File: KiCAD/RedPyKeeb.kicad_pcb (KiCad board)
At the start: 4 copper layers, 482.6 x 183.4 mm, 340 parts, among them J0 Conn_01x04, J1 Conn_01x04, K0,0 KEYSW, K0,1 KEYSW, K0,2 KEYSW, K0,3 KEYSW, K0,4 KEYSW, K0,5 KEYSW, K1,0 KEYSW, K1,1 KEYSW, K1,2 KEYSW, K1,3 KEYSW, K1,4 KEYSW, K1,5 KEYSW, K10,0 KEYSW, K10,1 KEYSW, K10,2 KEYSW, K10,3 KEYSW, K10,4 KEYSW, K10,5 KEYSW, K11,0 KEYSW, K11,1 KEYSW, K11,2 KEYSW, K11,3 KEYSW, K11,4 KEYSW, K11,5 KEYSW, K12,0 KEYSW, K12,1 KEYSW, K12,2 KEYSW, K12,3 KEYSW, K13,1 KEYSW, K13,2 KEYSW, K14,0 KEYSW, K14,1 KEYSW, K14,3 KEYSW, K14,6 KEYSW, K15,0 KEYSW, K15,1 KEYSW, K15,3 KEYSW, K15,5 KEYSW, K15,6 KEYSW, K16,0 KEYSW, K16,1 KEYSW, K16,3 KEYSW, K16,4 KEYSW, K16,5 KEYSW, K16,6 KEYSW, K17,0 KEYSW, K17,1 KEYSW, K17,3 KEYSW, K17,4 KEYSW, K17,5 KEYSW, K17,6 KEYSW, K18,0 KEYSW, K18,1 KEYSW, K18,3 KEYSW, K18,4 KEYSW, K18,5 KEYSW, K18,6 KEYSW, K19,0 KEYSW, K19,1 KEYSW, K19,3 KEYSW, K19,4 KEYSW, K19,6 KEYSW, K2,0 KEYSW, K2,1 KEYSW, K2,2 KEYSW, K2,3 KEYSW, K2,4 KEYSW, K2,5 KEYSW, K20,0 KEYSW, K20,1 KEYSW, K3,0 KEYSW, K3,1 KEYSW, K3,2 KEYSW, K3,3 KEYSW, K3,4 KEYSW, K3,5 KEYSW, K4,0 KEYSW, K4,1 KEYSW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

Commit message: Update KiCAD files.
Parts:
- added C4: 0805B101K100CT, Capacitor_SMD:C_0805_2012Metric_Pad1.18x1.45mm_HandSolder, B.Cu at (452.6, 82.5)
- added C5: 0805B101K100CT, Capacitor_SMD:C_0805_2012Metric_Pad1.18x1.45mm_HandSolder, B.Cu at (438.0, 80.3)
- added C7: 0805B101K100CT, Capacitor_SMD:C_0805_2012Metric_Pad1.18x1.45mm_HandSolder, B.Cu at (438.1, 75.0)
- added J2: Conn_01x04, Connector_JST:JST_EH_S4B-EH_1x04_P2.50mm_Horizontal, F.Cu at (442.1, 51.3)
- added R1: APC0805B1K00N, Resistors_SMD:R_0805_HandSoldering, B.Cu at (458.1, 81.9)
- added R2: APC0805B1K00N, Resistors_SMD:R_0805_HandSoldering, B.Cu at (460.1, 81.9)
- added R3: ERJ-6RED2003V, Resistors_SMD:R_0805_HandSoldering, B.Cu at (460.2, 78.5)
- added R4: APC0805B1K00N, Resistors_SMD:R_0805_HandSoldering, B.Cu at (458.5, 74.0)
- added R5: APC0805B1K00N, Resistors_SMD:R_0805_HandSoldering, B.Cu at (456.6, 74.0)
- C1, C2: moved to F.Cu
- C3: moved to B.Cu
- C6: value EEE-FK1A102AL -> EEE-FN1C102UV
- D0,0, D0,1, D0,2, D0,3, D0,4, D0,5, D1,0, D1,1, D1,2, D1,3, D1,4, D1,5, D10,0, D10,1, D10,2, D10,3, D10,4, D10,5, D11,0, D11,1, D11,2, D11,3, D11,4, D11,5, D12,0, D12,1, D12,3, D13,1, D13,2, D14,0, D14,1, D14,3, D14,6, D15,0, D15,1, D15,3, D15,5, D15,6, D16,0, D16,1, D16,3, D16,4, D16,5, D16,6, D17,0, D17,1, D17,3, D17,4, D17,5, D17,6, D18,0, D18,1, D18,3, D18,4, D18,5, D18,6, D19,0, D19,1, D19,3, D19,4, D19,6, D2,0, D2,1, D2,2, D2,3, D2,4, D2,5, D20,0, D20,1, D3,0, D3,1, D3,2, D3,3, D3,4, D3,5, D4,0, D4,1, D4,2, D4,3, D4,4, D5,0, D5,1, D5,2, D5,3, D5,4, D6,0, D6,1, D6,2, D6,3, D6,4, D7,0, D7,1, D7,2, D7,3, D7,4, D8,0, D8,1, D8,2, D8,3, D8,4, D8,5, D9,0, D9,1, D9,2, D9,3, D9,4, D9,5: value D -> BAT54W-HG3-08
- K0,0, K0,1, K0,2, K0,3, K0,4, K0,5, K1,0, K1,1, K1,2, K1,3, K1,4, K1,5, K10,0, K10,1, K10,2, K10,3, K10,4, K10,5, K11,0, K11,1, K11,2, K11,3, K11,4, K11,5, K12,0, K12,1, K12,2, K12,3, K13,1, K13,2, K14,0, K14,1, K14,3, K14,6, K15,0, K15,1, K15,3, K15,5, K15,6, K16,0, K16,1, K16,3, K16,4, K16,5, K16,6, K17,0, K17,1, K17,3, K17,4, K17,5, K17,6, K18,0, K18,1, K18,3, K18,4, K18,5, K18,6, K19,0, K19,1, K19,3, K19,4, K19,6, K2,0, K2,1, K2,2, K2,3, K2,4, K2,5, K20,0, K20,1, K3,0, K3,1, K3,2, K3,3, K3,4, K3,5, K4,0, K4,1, K4,2, K4,3, K4,4, K5,0, K5,1, K5,2, K5,3, K5,4, K6,0, K6,1, K6,2, K6,3, K6,4, K7,0, K7,1, K7,2, K7,3, K7,4, K8,0, K8,1, K8,2, K8,3, K8,4, K8,5, K9,0, K9,1, K9,2, K9,3, K9,4, K9,5: value KEYSW -> ~
- LD0,0, LD0,1, LD0,2, LD0,3, LD0,4, LD0,5, LD1,0, LD1,1, LD1,2, LD1,3, LD1,4, LD1,5, LD10,0, LD10,1, LD10,2, LD10,3, LD10,4, LD10,5, LD11,0, LD11,1, LD11,2, LD11,3, LD11,4, LD11,5, LD12,0, LD12,1, LD12,2, LD12,3, LD13,1, LD13,2, LD14,0, LD14,1, LD14,3, LD14,6, LD15,0, LD15,1, LD15,3, LD15,5, LD15,6, LD16,0, LD16,1, LD16,3, LD16,4, LD16,5, LD16,6, LD17,0, LD17,1, LD17,3, LD17,4, LD17,5, LD17,6, LD17,7, LD18,0, LD18,1, LD18,3, LD18,4, LD18,5, LD18,6, LD18,7, LD19,0, LD19,1, LD19,3, LD19,4, LD19,6, LD19,7, LD2,0, LD2,1, LD2,2, LD2,3, LD2,4, LD2,5, LD20,0, LD20,1, LD20,7, LD3,0, LD3,1, LD3,2, LD3,3, LD3,4, LD3,5, LD4,0, LD4,1, LD4,2, LD4,3, LD4,4, LD5,0, LD5,1, LD5,2, LD5,3, LD5,4, LD6,0, LD6,1, LD6,2, LD6,3, LD6,4, LD7,0, LD7,1, LD7,2, LD7,3, LD7,4, LD8,0, LD8,1, LD8,2, LD8,3, LD8,4, LD8,5, LD9,0, LD9,1, LD9,2, LD9,3, LD9,4, LD9,5: value APA102-2020 -> APA102 2020
- U0: value USB_Pico -> ~
- U10: value PCA9306DP -> PCA9306DQER; footprint Package_SO:SO-8_3.9x4.9mm_P1.27mm -> Package_SO:SSOP-8_2.95x2.8mm_P0.65mm
- moved U10 375.7 mm to (455.4, 79.4)
- moved U11 374.3 mm to (443.8, 78.7)
- moved U0 348.4 mm to (431.9, 67.1)
- moved C6 346.7 mm to (491.4, 73.0)
- moved J0 344.5 mm to (486.9, 60.4)
- moved J1 339.7 mm to (480.7, 80.6), turned to 180 degrees
- moved C2 334.7 mm to (409.2, 84.2)
- moved U2 332.3 mm to (405.7, 84.3), turned to 270 degrees
- moved U1 36.6 mm to (107.4, 112.3), turned to 180 degrees
- moved U3 34.5 mm to (83.8, 86.1), turned to 270 degrees
- moved C1 33.6 mm to (107.8, 114.3), turned to 270 degrees
- moved C3 24.8 mm to (80.4, 86.5)
- moved K20,0 22.7 mm to (501.3, 102.5)
- moved LD20,0 22.7 mm to (501.3, 95.7)
- moved D17,0 22.7 mm to (435.6, 103.7)
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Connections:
- U10 pad 7: MAIN_VBUS -> Net-(C4-Pad2)
- U10 pad 8: MAIN_VBUS -> Net-(C4-Pad2)
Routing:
- net MAIN_VBUS: track 4476.7 -> 4998.0 mm, vias 47 -> 57
- net KEY_COL16: track 594.8 -> 181.5 mm
- net KEY_COL20: track 558.3 -> 149.0 mm
- net KEY_COL19: track 621.8 -> 214.2 mm
- net KEY_COL18: track 605.4 -> 200.1 mm
- net KEY_COL17: track 594.2 -> 190.0 mm
- net I2C_SDA0: track 60.3 -> 450.4 mm, vias 3 -> 5
- net I2C_SCL0: track 59.1 -> 447.0 mm, vias 4 -> 5
- net GNDPWR: track 3230.2 -> 3610.8 mm, vias 6 -> 9
- net PICO_33_REF: track 125.0 -> 497.8 mm, vias 1 -> 3
- net KEY_COL15: track 527.8 -> 178.2 mm
- net IO_INT0: track 46.6 -> 371.8 mm, vias 2 -> 4
- net KEY_COL14: track 507.4 -> 187.7 mm
- net IO_INT1: track 50.7 -> 367.3 mm, vias 2 -> 4
- net KEY_COL12: track 406.3 -> 146.0 mm, vias 2 -> 0
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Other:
- board size 482.6 x 183.4 mm -> 448.3 x 179.1 mm
- net class USB added: clearance 0.2, trace_width 0.4, via_dia 0.8, via_drill 0.4

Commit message: Update firmware and KiCAD files.
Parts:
- D12,2: value BAT54W-HG3-18 -> BAT54W-HG3-08
- J2: footprint Connector_JST:JST_EH_S4B-EH_1x04_P2.50mm_Horizontal -> Connector_JST:JST_EH_S7B-EH_1x07_P2.50mm_Horizontal
- U10: value PCA9306DQER -> PCA9306DP
- moved J2 2.95 mm to (445.0, 50.9)
- moved LD13,2 1.03 mm to (353.3, 140.7)
- moved LD0,4 1.03 mm to (100.2, 179.9)
- moved LD19,1 0.50 mm to (482.1, 121.5)
- moved LD0,2 0.35 mm to (93.1, 140.7)
- moved LD19,0 0.24 mm to (482.0, 95.6)
- moved LD17,0 0.12 mm to (443.4, 95.6)
- moved LD18,0 0.12 mm to (462.7, 95.6)
- moved LD20,0 0.11 mm to (501.3, 95.6)
- moved LD17,3 0.10 mm to (443.5, 140.7)
- moved LD18,3 0.10 mm to (462.8, 140.7)
- moved LD19,3 0.10 mm to (482.1, 140.7)
- moved LD0,0 0.08 mm to (88.5, 95.5)
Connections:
- U0 pad 21: Net-(J2-Pad4) -> Net-(U0-Pad21)
- U0 pad 22: Net-(J2-Pad3) -> Net-(J2-Pad5)
- U0 pad 24: Net-(J2-Pad2) -> Net-(J2-Pad3)
- U0 pad 25: Net-(J2-Pad1) -> Net-(J2-Pad4)
- U0 pad 26: Net-(U0-Pad26) -> Net-(J2-Pad6)
- U0 pad 27: Net-(U0-Pad27) -> Net-(J2-Pad7)
- U0 pad 36: Net-(U0-Pad36) -> Net-(J2-Pad1)
- U0 pad 38: Net-(U0-Pad38) -> Net-(J2-Pad2)
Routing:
- net MAIN_VBUS: track 4998.0 -> 4783.6 mm, vias 57 -> 56
- net GNDPWR: track 3610.8 -> 3540.1 mm
- net Net-(J2-Pad2): track 4.13 -> 37.3 mm
- net Net-(J2-Pad7): track 0.00 -> 28.9 mm
- net Net-(J2-Pad1): track 4.82 -> 29.0 mm
- net Net-(J2-Pad6): track 0.00 -> 24.1 mm
- net Net-(LD16,3-Pad2): track 30.4 -> 22.2 mm
- net Net-(J2-Pad5): track 0.00 -> 3.54 mm
- net Net-(J2-Pad4): track 4.11 -> 7.24 mm
- net Net-(LD17,0-Pad3): track 16.2 -> 17.6 mm
- net Net-(LD14,3-Pad3): track 16.2 -> 17.6 mm
- net Net-(LD14,1-Pad3): track 16.2 -> 17.6 mm
- net Net-(LD10,5-Pad4): track 21.1 -> 22.5 mm
- net Net-(LD7,2-Pad3): track 16.2 -> 17.6 mm
- net Net-(LD18,6-Pad3): track 19.6 -> 21.0 mm
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
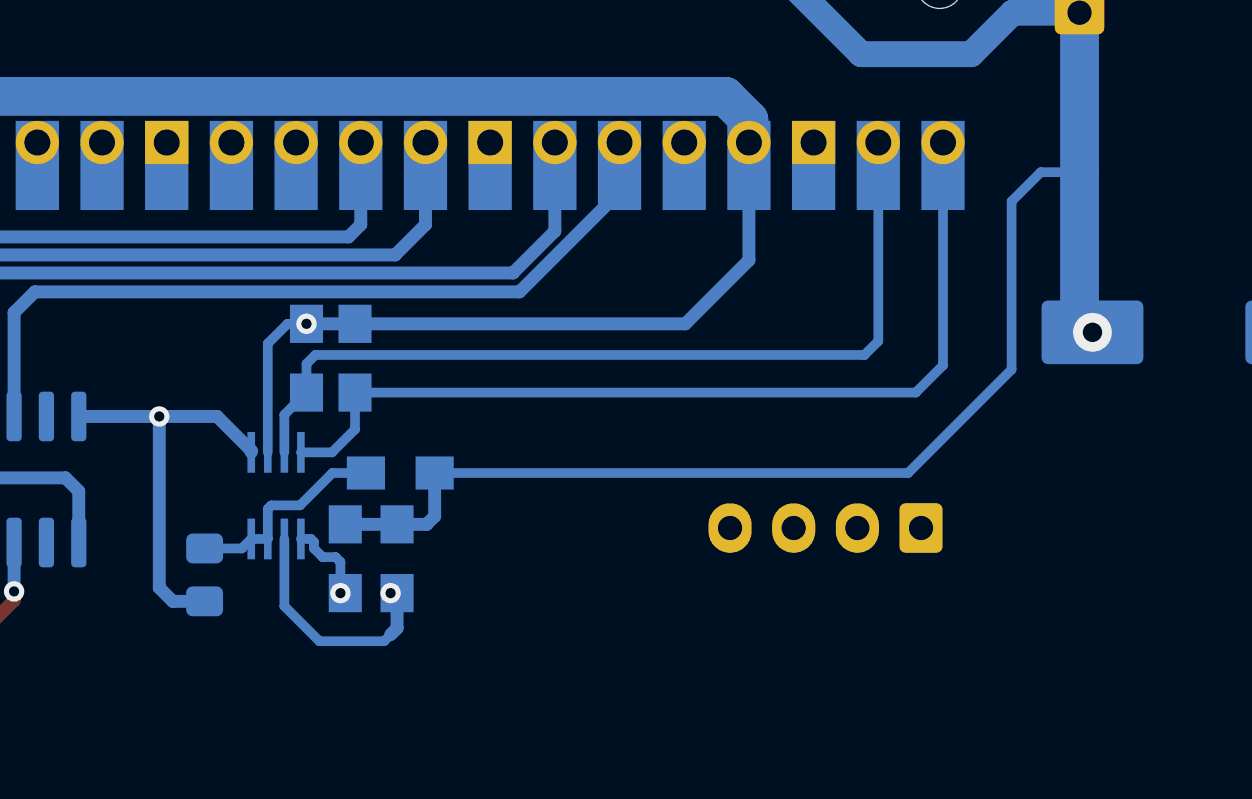
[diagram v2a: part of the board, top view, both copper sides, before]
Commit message: Update KiCAD files.
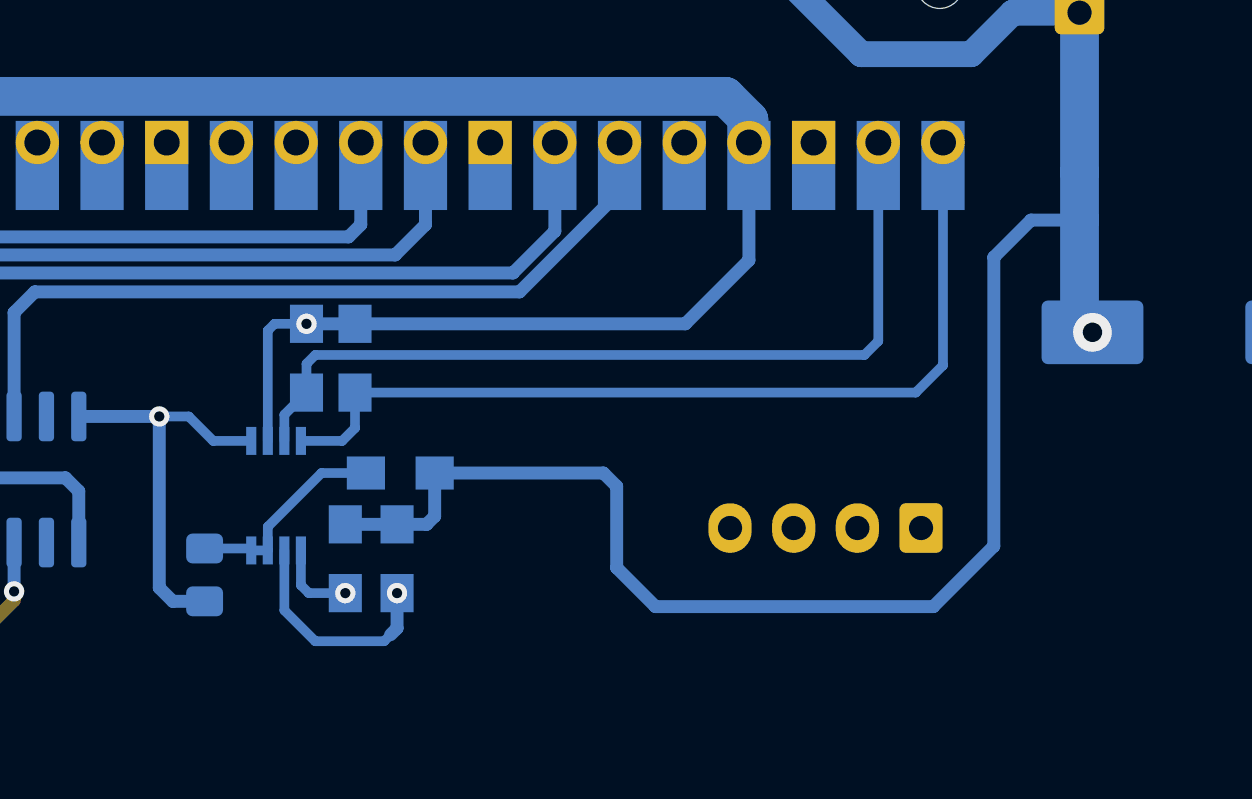
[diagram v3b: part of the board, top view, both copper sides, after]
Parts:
- U10: value PCA9306DP -> PCA9306DP,118; footprint Package_SO:SSOP-8_2.95x2.8mm_P0.65mm -> Package_SO:TSSOP-8_3x3mm_P0.65mm
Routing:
- net MAIN_VBUS: track 4783.6 -> 4795.4 mm
- net GNDPWR: track 3540.1 -> 3543.4 mm
